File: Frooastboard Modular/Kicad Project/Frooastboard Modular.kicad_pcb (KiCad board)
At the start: 4 copper layers, 44.6 x 28.3 mm, 46 parts, among them J1 Conn_01x08, J10 Conn_01x02, J2 Conn_01x06, J3 Conn_01x06, J4 Conn_01x10, J5 Conn_01x12, J6 SW Interface, J7 Conn_01x04, J8 Conn_01x08, J9 Conn_01x05, U1 IS31FL3733-QF, U2 RP2040, U3 W25Q32JVZP, U4 LM317L_SOT-89, Y1 12MHz

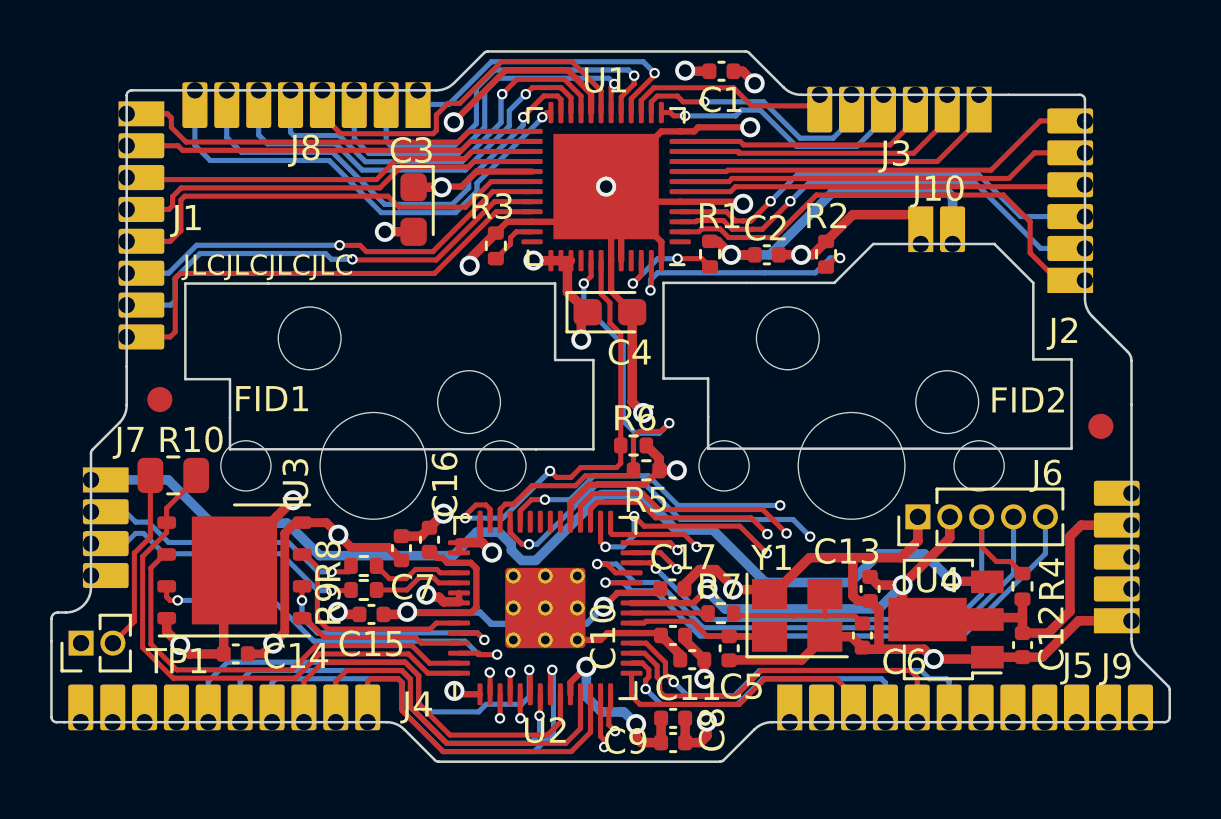
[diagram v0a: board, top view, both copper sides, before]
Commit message: some stuff
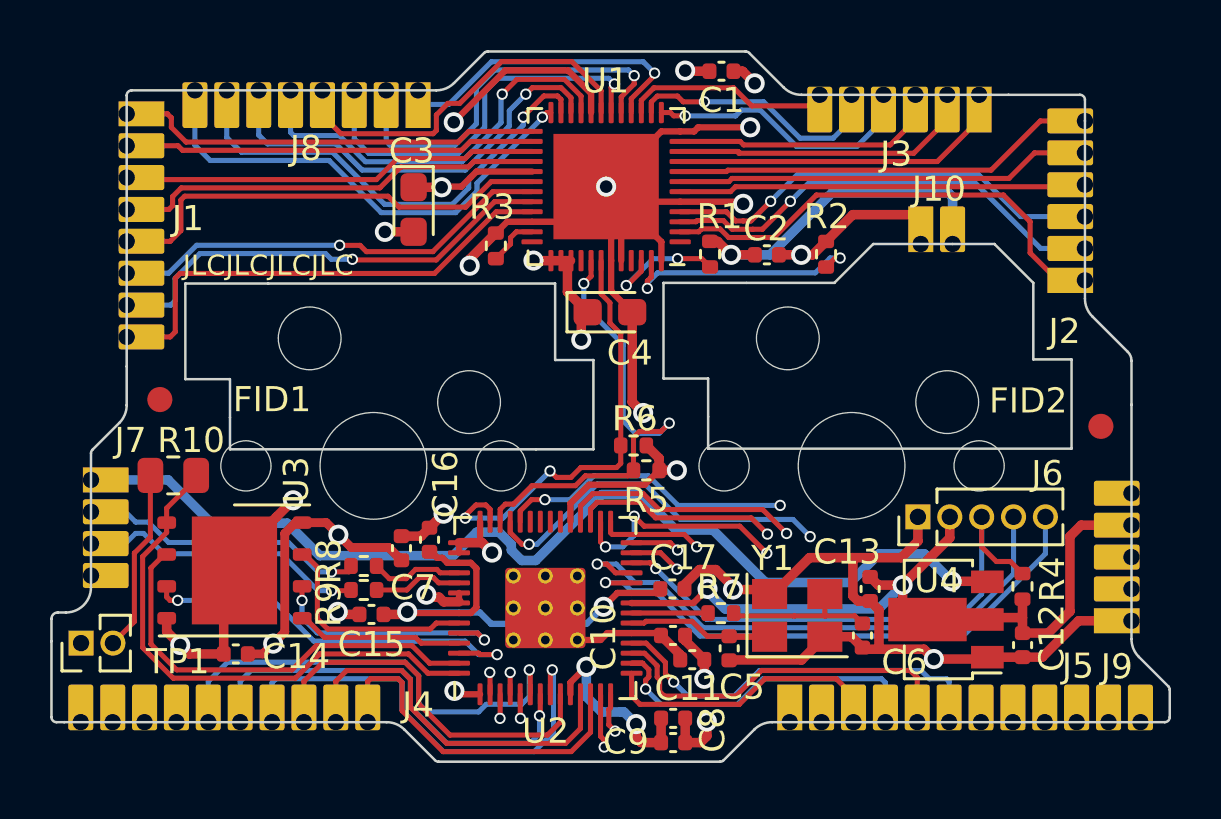
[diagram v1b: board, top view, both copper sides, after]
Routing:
- net Net-(U1-~{SDB}): track 4.67 -> 5.17 mm
